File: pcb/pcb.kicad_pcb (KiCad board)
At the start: 2 copper layers, 100 x 100 mm, 45 parts, among them J1 NMJ4HCD2, J2 NMJ4HCD2, J3 694106301002, SW1 FSWITCH, U1 RC4558, U2 L78L09_TO92

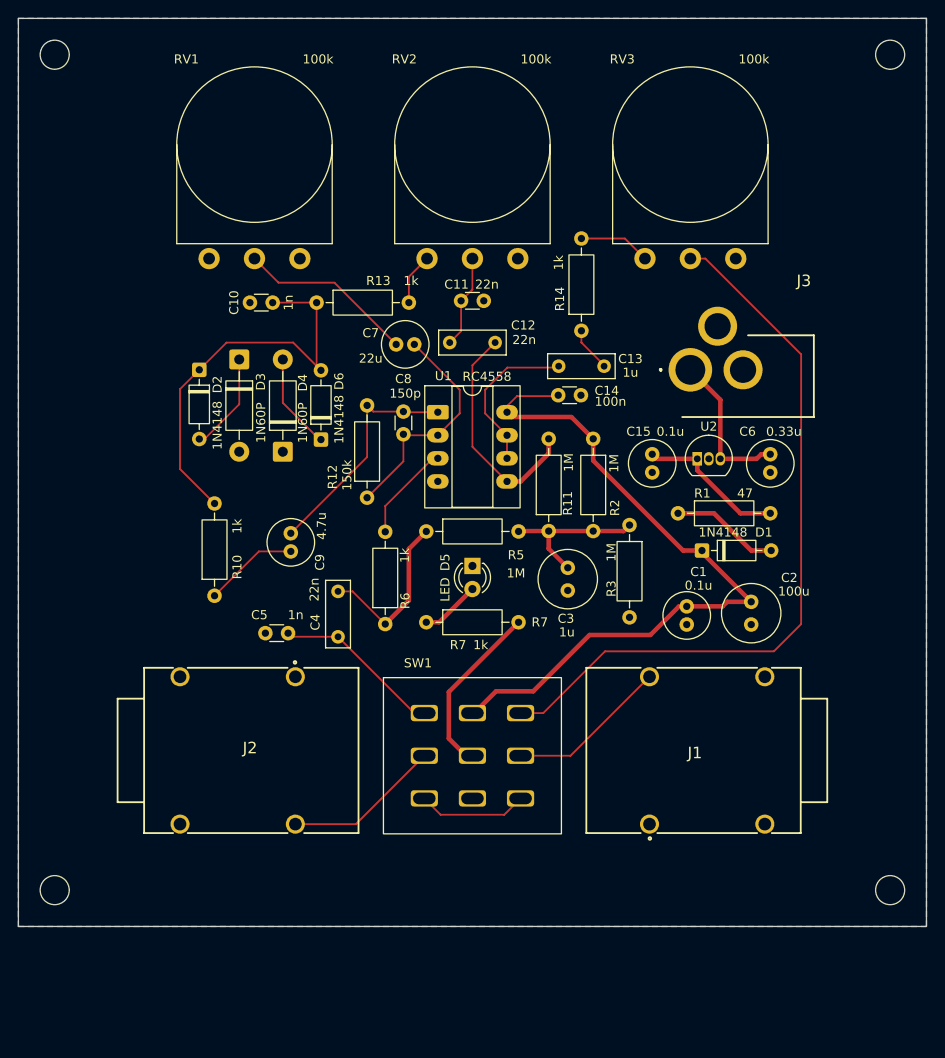
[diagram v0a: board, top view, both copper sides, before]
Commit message: 1590b pcb
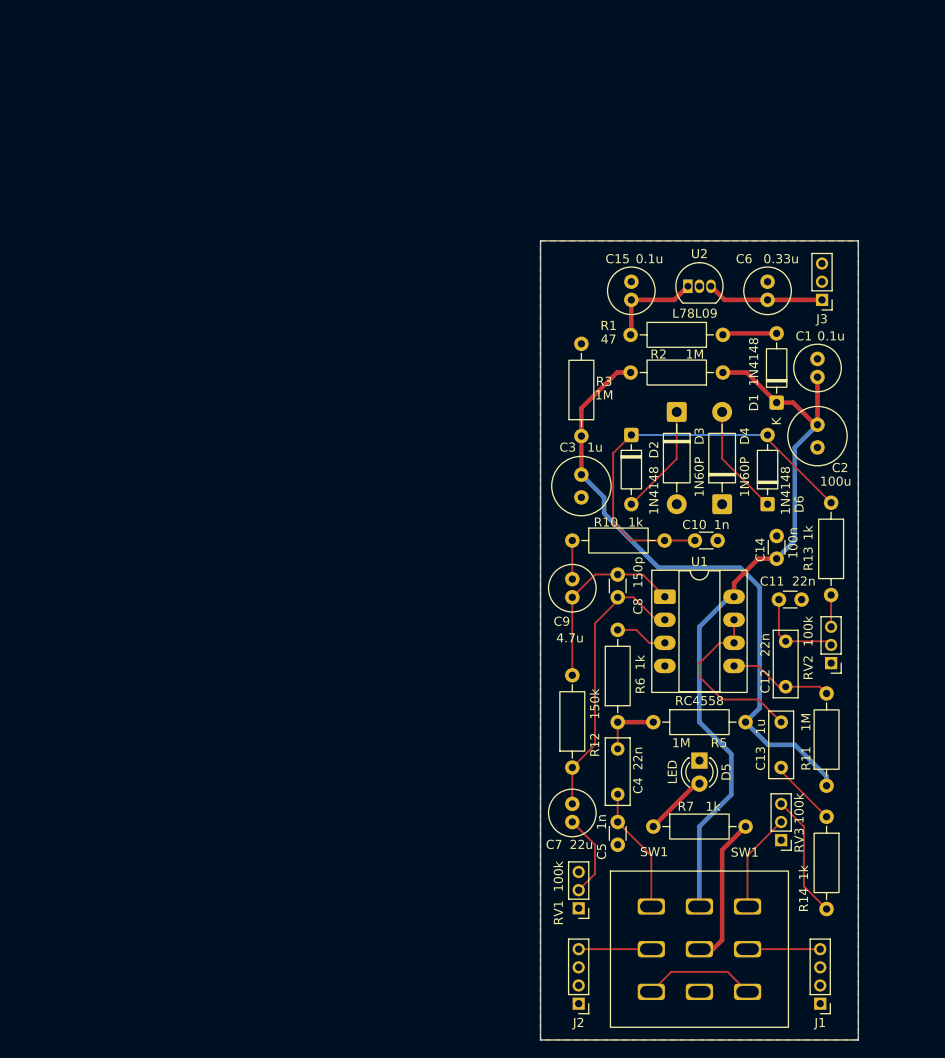
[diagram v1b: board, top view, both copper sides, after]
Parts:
- removed REF** (x4): MountingHole_3.2mm_M3, MountingHole:MountingHole_3.2mm_M3
- J1, J2: footprint NMJ4HCD2:NMJ4HCD2 -> Connector_PinHeader_2.00mm:PinHeader_1x04_P2.00mm_Vertical
- J3: footprint PowerJackFemale:694106301002 -> Connector_PinHeader_2.00mm:PinHeader_1x03_P2.00mm_Vertical
- RV1, RV2, RV3: footprint Potentiometer_THT:Potentiometer_Omeg_PC16BU_Vertical -> Connector_PinHeader_2.00mm:PinHeader_1x03_P2.00mm_Vertical
- U2: value L78L09_TO92 -> L78L09
- moved RV1 77.9 mm to (161.7, 135.5), turned to 180 degrees
- moved RV3 64.2 mm to (184.0, 128.0), turned to 180 degrees
- moved R13 60.8 mm to (189.5, 90.8), turned to -90 degrees
- moved R14 59.9 mm to (189.0, 125.4), turned to -90 degrees
- moved C10 57.8 mm to (177.0, 95.0), turned to 180 degrees
- moved RV2 56.3 mm to (189.5, 108.5), turned to 180 degrees
- moved C7 56.1 mm to (161.0, 126.0), turned to 90 degrees
- moved J2 55.4 mm to (161.7, 146.0)
- moved D6 49.7 mm to (182.5, 91.0)
- moved C12 49.5 mm to (184.5, 106.1), turned to -90 degrees
- moved D4 48.7 mm to (177.5, 91.0)
- moved D3 48.5 mm to (172.5, 80.8)
- moved D2 48.1 mm to (167.5, 83.4)
- moved C11 48.0 mm to (183.8, 101.5)
- moved C13 46.2 mm to (184.0, 115.0), turned to -90 degrees
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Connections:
- RV1 pad 3: unconnected-(RV1-Pad3) -> GND
- RV2 pad 1: unconnected-(RV2-Pad1) -> GND
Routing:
- net /VVOLOUT: track 81.2 -> 10.8 mm
- net /VBIAS: track 17.4 -> 68.1 mm
- net /AMP2+: track 25.4 -> 11.4 mm
- net Net-(C4-Pad2): track 18.8 -> 6.87 mm
- net Net-(C7-Pad1): track 19.5 -> 9.28 mm
- net /VOUT: track 17.8 -> 8.00 mm
- net /VIN: track 17.3 -> 8.00 mm
- net Net-(C9-Pad2): track 10.4 -> 4.25 mm
- net Net-(D1-A): track 12.0 -> 5.99 mm
- net Net-(R14-Pad2): track 7.92 -> 13.7 mm
- net /V9: track 16.4 -> 10.7 mm
- net /AMP1-: track 25.6 -> 31.0 mm
- net /AMP1+: track 10.8 -> 5.78 mm
- net /AMP1OUT: track 25.7 -> 20.8 mm
- net /VAMPIN: track 18.6 -> 13.9 mm
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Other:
- board size 100 x 100 mm -> 35 x 88 mm
- board text removed: "RV1"
